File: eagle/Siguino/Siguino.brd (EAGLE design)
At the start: 76 x 38.5 mm, 48 parts, among them J1 FTDI, J4 10118193-0001LF, Q1 MOSFET P-CH 20V 5.3A SOT-23, Q2 MOSFET P-CH 20V 5.3A SOT-23, U1 ATMEGA328P_TQFP, U2 LIS3MDLTR_LIS3MDLTR, U3 SPARKFUN-SENSORS_LIS3DH, U4 BME280, U5 FT232RL, U6 MAX1724EZK33+T, Y1 8MHz

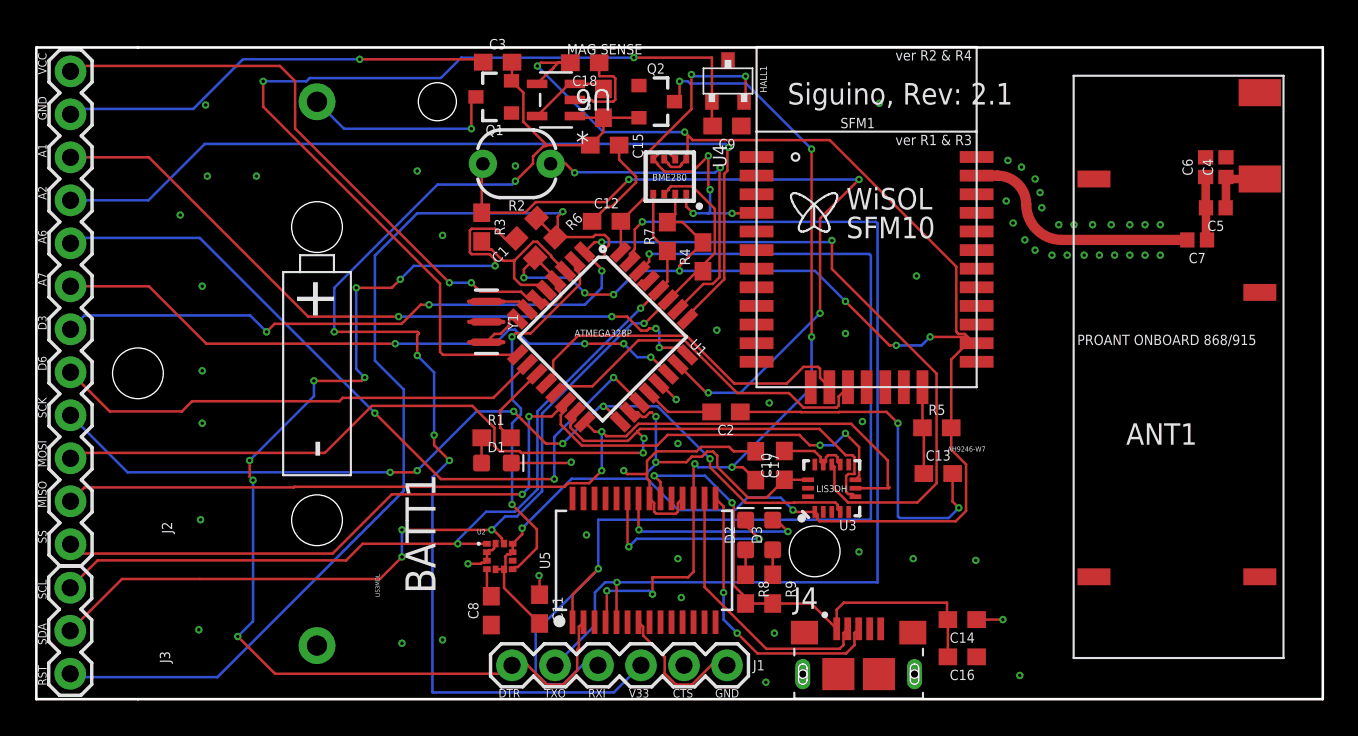
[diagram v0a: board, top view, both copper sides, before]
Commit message: ufl
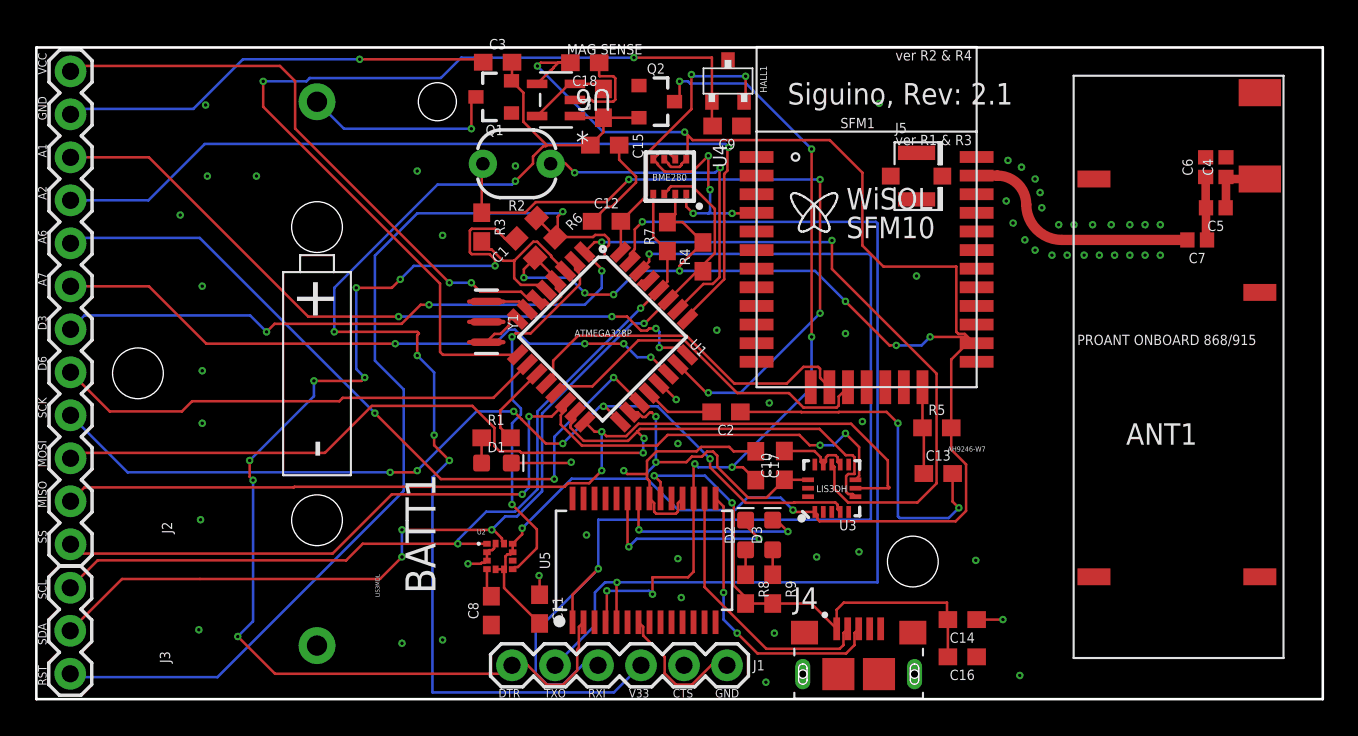
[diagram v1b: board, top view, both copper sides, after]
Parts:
- added J5: U.FL, SparkFun-Connectors:U.FL
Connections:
- removed net CTS: J1.5
- removed net N$6: C7.2, SFM1.30
- new net WISOL_ANT: C7.2, J5.FEED, SFM1.30
- net GND: now also J1.5, J5.1, J5.2
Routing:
- net WISOL_ANT: track 0.00 -> 14.0 mm
- net N$6: track 14.0 -> 0.00 mm
- net LIGHT_SENSE: track 45.9 -> 42.7 mm
- net VCC: track 185.6 -> 188.1 mm
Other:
- outline, holes or cut-outs redrawn
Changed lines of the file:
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@@
 <plain>
 <text x="44.38" y="35.13" size="1.27" layer="21">Siguino, Rev: 2.1</text>
-<wire x1="0" y1="0" x2="6" y2="0" width="0.1524" layer="20"/>
-<wire x1="6" y1="0" x2="76" y2="0" width="0.1524" layer="20"/>
+<wire x1="0" y1="0" x2="76" y2="0" width="0.1524" layer="20"/>
 <wire x1="76" y1="0" x2="76" y2="38.5" width="0.1524" layer="20"/>
-<wire x1="76" y1="38.5" x2="6" y2="38.5" width="0.1524" layer="20"/>
-<wire x1="6" y1="38.5" x2="0" y2="38.5" width="0.1524" layer="20"/>
+<wire x1="76" y1="38.5" x2="0" y2="38.5" width="0.1524" layer="20"/>
 <wire x1="0" y1="38.5" x2="0" y2="0" width="0.1524" layer="20"/>
-<hole x="45.98" y="8.73" drill="3"/>
+<hole x="51.78" y="8.13" drill="3"/>
 <text x="37.6" y="0.1" size="0.5" layer="21">CTS</text>
 <text x="40.1" y="0.1" size="0.5" layer="21">GND</text>
@@
 <attribute name="PROD_ID" value="SI2323DDS-T1-GE3" x="36.6" y="35.3" size="1.778" layer="27" rot="R270" display="off"/>
 </element>
+<element name="J5" library="SparkFun-Connectors" package="U.FL" value="U.FL" x="52" y="30.9" smashed="yes">
+<attribute name="NAME" x="50.73" y="33.44" size="0.6096" layer="25" font="vector" ratio="20"/>
+<attribute name="PROD_ID" value="CONN-09193" x="52" y="30.9" size="1.778" layer="27" display="off"/>
+<attribute name="SF_ID" value="WRL-09144" x="52" y="30.9" size="1.778" layer="27" display="off"/>
+<attribute name="VALUE" x="50.73" y="28.36" size="0.6096" layer="27" font="vector" ratio="20" align="top-left"/>
+</element>
 </elements>
 <signals>
@@
 <via x="34.7" y="13.5" extent="1-16" drill="0.2"/>
 <via x="47.8" y="21.6" extent="1-16" drill="0.2"/>
-<via x="51.8" y="8.3" extent="1-16" drill="0.2"/>
+<via x="46.1" y="8.4" extent="1-16" drill="0.2"/>
 <via x="55.5" y="8.2" extent="1-16" drill="0.2"/>
 <via x="21.6" y="3.3" extent="1-16" drill="0.2"/>
@@
 <wire x1="36.76816875" y1="18.647515625" x2="36.852484375" y2="18.647515625" width="0.1524" layer="1"/>
 <wire x1="36.852484375" y1="18.647515625" x2="37.8" y2="17.7" width="0.1524" layer="1"/>
+<contactref element="J5" pad="2"/>
+<contactref element="J5" pad="1"/>
+<contactref element="J1" pad="5"/>
 </signal>
 <signal name="VCC">
@@
 <wire x1="54.8512" y1="21.5788" x2="55.4" y2="21.03" width="0.1524" layer="1"/>
 <wire x1="54.3488" y1="25.55394375" x2="54.3488" y2="21.6966625" width="0.1524" layer="1"/>
-<wire x1="46.87654375" y1="33.0262" x2="54.3488" y2="25.55394375" width="0.1524" layer="1"/>
 <wire x1="39.38" y1="26.98" x2="38" y2="25.6" width="0.1524" layer="1"/>
 <wire x1="38" y1="25.6" x2="38" y2="25.3" width="0.1524" layer="1"/>
@@
 <wire x1="36.599996875" y1="16.695" x2="36.6" y2="16.695" width="0.1524" layer="1"/>
 <wire x1="54.05" y1="14.7445375" x2="54.05" y2="16.03" width="0.1524" layer="1"/>
+<wire x1="46.87654375" y1="33.0262" x2="48.8" y2="31.10274375" width="0.1524" layer="1"/>
+<wire x1="48.8" y1="31.10274375" x2="48.8" y2="26.8" width="0.1524" layer="1"/>
+<wire x1="48.8" y1="26.8" x2="50.04605625" y2="25.55394375" width="0.1524" layer="1"/>
+<wire x1="50.04605625" y1="25.55394375" x2="54.3488" y2="25.55394375" width="0.1524" layer="1"/>
 </signal>
 <signal name="N$2">
@@
 <wire x1="28.87835625" y1="28.74" x2="29.503053125" y2="29.364696875" width="0.1524" layer="1"/>
 <wire x1="29.503053125" y1="29.364696875" x2="33.664696875" y2="29.364696875" width="0.1524" layer="1"/>
-<wire x1="35" y1="30.7" x2="48.6" y2="30.7" width="0.1524" layer="16"/>
-<via x="48.6" y="30.7" extent="1-16" drill="0.2"/>
-<wire x1="48.6" y1="30.7" x2="46.3" y2="28.4" width="0.1524" layer="1"/>
-<wire x1="46.3" y1="28.4" x2="46.3" y2="22.8" width="0.1524" layer="1"/>
+<wire x1="35" y1="30.7" x2="46.3" y2="30.7" width="0.1524" layer="16"/>
+<via x="46.3" y="30.7" extent="1-16" drill="0.2"/>
+<wire x1="46.3" y1="30.7" x2="46.3" y2="22.8" width="0.1524" layer="1"/>
 <via x="46.3" y="22.8" extent="1-16" drill="0.2"/>
 <wire x1="46.3" y1="22.8" x2="41.6" y2="18.1" width="0.1524" layer="16"/>
@@
 <wire x1="24.017190625" y1="20.344571875" x2="23.8497625" y2="20.512" width="0.1524" layer="1"/>
 </signal>
-<signal name="N$6">
+<signal name="WISOL_ANT">
 <contactref element="SFM1" pad="30"/>
 <contactref element="C7" pad="2"/>
@@
 <wire x1="60.58" y1="27.13" x2="68" y2="27.13" width="0.6096" layer="1"/>
 <wire x1="55.55" y1="30.93" x2="56.78" y2="30.93" width="0.6096" layer="1"/>
+<contactref element="J5" pad="FEED"/>
+<wire x1="53.525" y1="30.9" x2="55.55" y2="30.93" width="0" layer="19" extent="1-1"/>
 </signal>
 <signal name="5V">
@@
 <wire x1="42.6" y1="2.7" x2="47.8345375" y2="2.7" width="0.1524" layer="1"/>
 </signal>
-<signal name="CTS">
-<contactref element="J1" pad="5"/>
-</signal>
 <signal name="N$17">
